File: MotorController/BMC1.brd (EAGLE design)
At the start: 92 x 50 mm, 58 parts, among them IC2 LP2950, IC3 MEGA8-AI, Q1 20MHz, U1 BTN8982TA, U2 BTN8982TA, U3 BTN8982TA, U4 TC77-5.0MCTTR, U5 MCP2561-E/SN

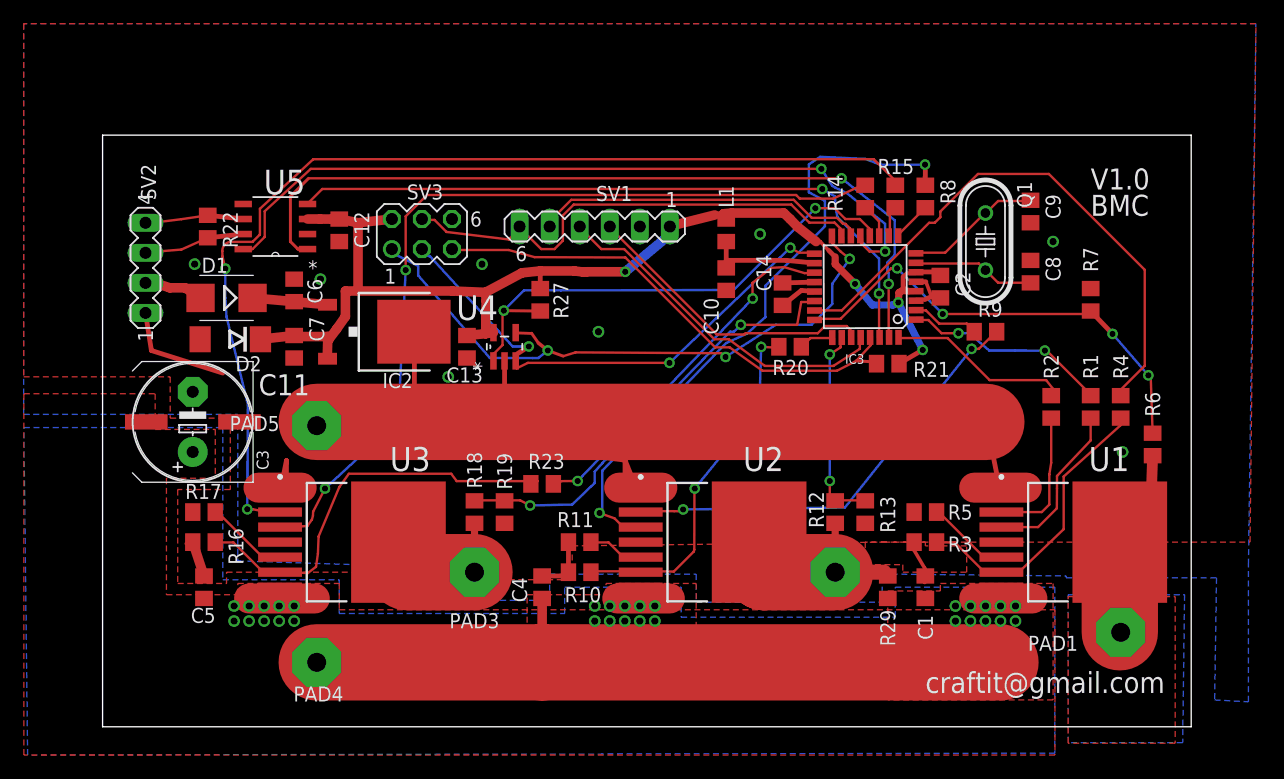
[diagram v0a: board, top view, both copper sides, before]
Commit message: Finished version 1.
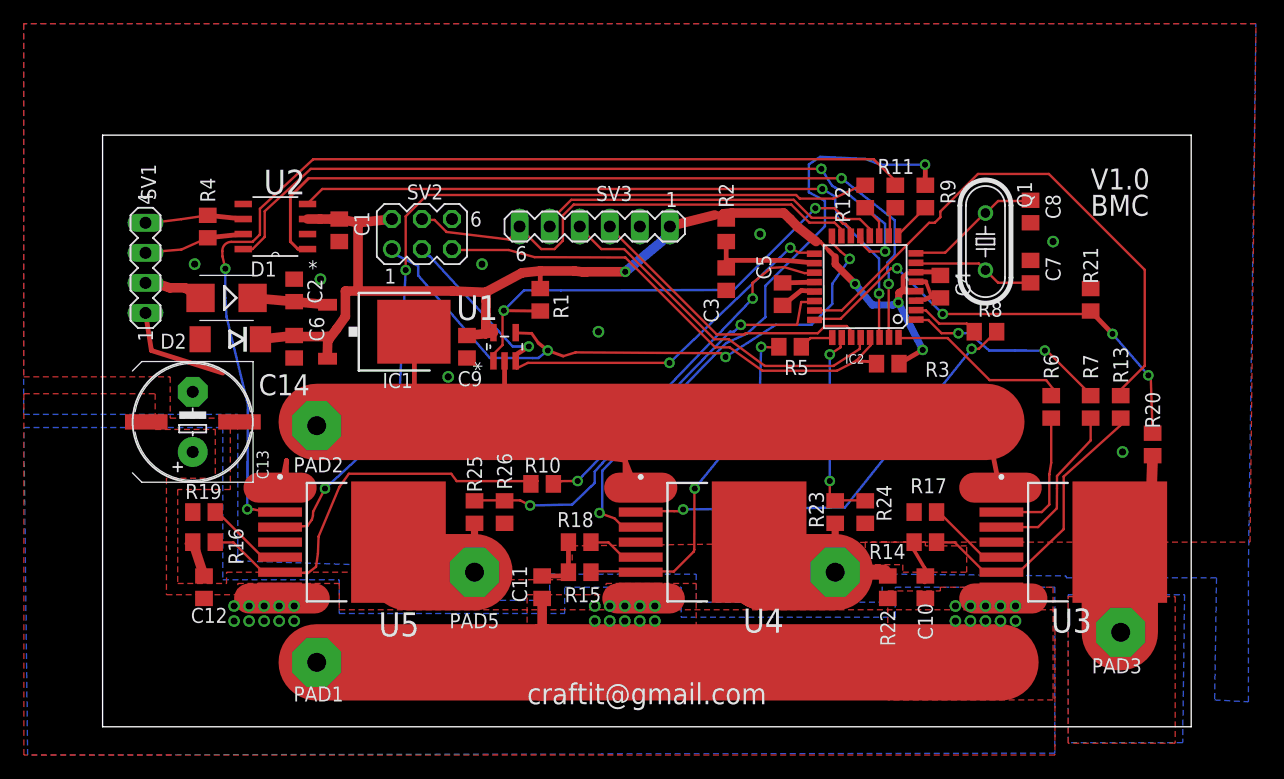
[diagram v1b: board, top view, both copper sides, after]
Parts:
- removed IC3: MEGA8-AI, atmel:TQFP32-08
- removed L1: 10uH, resistor:R0805
- removed R27, R29: 10k, resistor:R0805
- added IC1: LP2950, linear:DPACK
- added R24, R26: 1k, resistor:R0805
- added R25: 30k, resistor:R0805
- C1, C4, C5: value 0.1uf 40v -> 0.1uf
- C10, C12: value 0.1uf -> 0.1uf 40v
- C11: value (none) -> 0.1uf 40v; device resistor:E5-10,5 -> rcl:C0805
- C13: value 0.1uf -> 1000uF 50V; device rcl:C0805 -> rcl:UD-10X10_NICHICON
- C14: value 0.1uf -> 1000uf 50V; device rcl:C0805 -> resistor:E5-10,5
- C2: value 0.1uf -> 10uf 35V
- C3: value 1000uF 40V -> 0.1uf; device rcl:UD-10X10_NICHICON -> rcl:C0805
- C6: value 10uf 35V -> 2.2uf 10V
- C7: value 2.2uf 10V -> 18pf
- C9: value 18pf -> 0.1uf
- IC2: value LP2950 -> MEGA8-AI; device linear:DPACK -> atmel:TQFP32-08
- R10, R3: value 750R -> 10k
- R11, R5: value 100R -> 10k
- R12, R6: value 30k -> 10k
- R13, R7: value 1k -> 10k
- R14, R15: value 10k -> 750R
- R18: value 30k -> 100R
- R19: value 1k -> 100R
- R2: value 10k -> 10uH
- R20, R23: value 10k -> 30k
- R21: value 10k -> 1k
- R22: value 120R -> 10k
- R4: value 10k -> 120R
- SV1: device con-lstb:MA06-1 -> con-lstb:MA04-1
- SV2: device con-lstb:MA04-1 -> con-lstb:MA03-2
- SV3: device con-lstb:MA03-2 -> con-lstb:MA06-1
- U1: value BTN8982TA -> TC77-5.0MCTTR; device BTN8982TA:TO127P1500X440-8N-1 -> temp-tc77-5v:SOT95P290X145-5N
- U2: value BTN8982TA -> MCP2561-E/SN; device BTN8982TA:TO127P1500X440-8N-1 -> Microchip-MCP2561-E_SN:SOIC127P600X175-8N
- U4: value TC77-5.0MCTTR -> BTN8982TA; device temp-tc77-5v:SOT95P290X145-5N -> BTN8982TA:TO127P1500X440-8N-1
- U5: value MCP2561-E/SN -> BTN8982TA; device Microchip-MCP2561-E_SN:SOIC127P600X175-8N -> BTN8982TA:TO127P1500X440-8N-1
- moved R4 78.6 mm to (8.89, 42.3)
- moved PAD1 68.0 mm to (18.1, 5.45)
- moved R22 65.1 mm to (66.4, 11.8)
- moved C7 62.6 mm to (78.4, 38.5)
- moved U3 61.0 mm to (81.0, 15.6)
- moved R17 61.0 mm to (69.5, 18.1)
- moved C1 58.0 mm to (20.0, 42.0), turned to 270 degrees
- moved PAD3 54.8 mm to (86.0, 7.99)
- moved C5 54.8 mm to (57.5, 36.6), turned to 270 degrees
- moved C2 54.6 mm to (16.2, 36.9), turned to 90 degrees
- moved C14 51.0 mm to (7.62, 25.8), turned to 90 degrees
- moved U1 49.8 mm to (34.0, 32.1), turned to 90 degrees
- moved C9 49.0 mm to (30.8, 32.1), turned to 270 degrees
- moved R1 47.4 mm to (37.0, 36.1), turned to 90 degrees
- moved C3 46.7 mm to (52.7, 37.8), turned to 270 degrees
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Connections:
- removed net N$1 (its old number): R5.2, U1.5
- new net N$14: R19.2, U5.5
- net +7V: now also SV1.2; no longer SV2.2
- net 18V: now also C10.1, C11.1, C12.1, C13.+, C14.+, PAD1.1, R22.2, U4.7, U5.7; no longer C1.1, C11.+, C3.+, C4.1, C5.1, PAD4.1, R29.2, U1.7, U2.7
- net GND: now also C11.2, C13.-, C14.-, C3.2, C7.1, C9.2, IC1.2, IC2.21, IC2.3, IC2.5, PAD2.1, R14.1, R15.1, R18.1, R21.1, R24.1, R26.1, SV1.1, SV2.6, SV3.2, U1.2, U2.2, U4.1, U5.1; no longer C11.-, C13.2, C14.2, C3.-, C7.2, C9.1, IC2.2, IC3.21, IC3.3, IC3.5, PAD5.1, R10.1, R11.1, R13.1, R3.1, R5.1, R7.1, SV1.2, SV2.1, SV3.6, U1.1, U2.1, U4.2, U5.2
- net N$10: now also R8.2, U4.2; no longer R9.2, U2.2
- net N$11: now also IC2.25, R5.1; no longer IC3.25, R20.1
- net N$12: now also IC2.2, R8.1; no longer IC3.2, R9.1
- net N$13: now also PAD5.1, R25.2, U5.8; no longer PAD3.1, R18.2, U3.8
- net N$15: now also R12.2, U5.3; no longer R14.2, U3.3
- net N$16: now also R11.2, U5.2; no longer R15.2, U3.2
- net N$17: now also IC2.19, R10.1; no longer IC3.19, R23.1
- net N$18: now also IC2.22, R25.1, R26.2; no longer IC3.22, R18.1, R19.2
- net N$19: now also R4.1, SV1.4, U2.6; no longer R22.1, SV2.4, U5.6
- net N$2: now also PAD3.1, R20.2, U3.8; no longer PAD1.1, R6.2, U1.8
- net N$21: now also IC2.9, R9.1; no longer IC3.9, R8.1
- net N$22: now also IC2.26, R23.1, R24.2; no longer IC3.26, R12.1, R13.2
- net N$23: now also R4.2, SV1.3, U2.7; no longer R22.2, SV2.3, U5.7
- net N$25: now also IC2.13, U2.8; no longer IC3.13, U5.8
- net N$26: now also C2.1, IC1.1; no longer C6.1, IC2.1
- net N$27: now also C7.2, IC2.7; no longer C8.2, IC3.7
- net N$3: now also R7.2, U3.3; no longer R1.2, U1.3
- net N$31: now also C8.2, IC2.8; no longer C9.2, IC3.8
- net N$32: now also IC2.15, SV2.4, SV3.6; no longer IC3.15, SV1.6, SV3.4
- net N$33: now also IC2.32, R6.1; no longer IC3.32, R2.1
- net N$34: now also IC2.17, SV2.3, U1.3; no longer IC3.17, SV3.3, U4.3
- net N$36: now also R15.2, R5.2, U4.6; no longer R10.2, R20.2, U2.6
- net N$37: now also IC2.27, SV3.3; no longer IC3.27, SV1.3
- net N$38: now also R13.2, R14.2, U3.6; no longer R3.2, R4.2, U1.6
- net N$39: now also R10.2, U5.6; no longer R23.2, U3.6
- net N$4: now also R6.2, U3.2; no longer R2.2, U1.2
- net N$40: now also C3.1, IC2.18, R2.1; no longer C10.1, IC3.18, L1.1
- net N$41: now also IC2.28, SV3.4; no longer IC3.28, SV1.4
- net N$42: now also IC2.30, U2.4; no longer IC3.30, U5.4
- net N$43: now also IC2.31, U2.1; no longer IC3.31, U5.1
- net N$44: now also IC2.11, R12.1; no longer IC3.11, R14.1
- net N$45: now also IC2.10, R11.1; no longer IC3.10, R15.1
- net N$46: now also IC2.1, R7.1; no longer IC3.1, R1.1
- net N$49: now also IC2.14, SV3.5; no longer IC3.14, SV1.5
- net N$5: now also IC2.24, R20.1, R21.2; no longer IC3.24, R6.1, R7.2
- net N$50: now also IC2.12, R1.1, U1.1; no longer IC3.12, R27.1, U4.1
- net N$52: now also IC2.29, R3.2, SV2.5; no longer IC3.29, R21.2, SV3.5
- net N$54: now also C5.1, IC2.20; no longer C14.1, IC3.20
- net N$55: now also IC2.23, R13.1; no longer IC3.23, R4.1
- net N$6: now also IC2.16, SV2.1, U1.4; no longer IC3.16, SV3.1, U4.4
- net N$7: now also PAD4.1, R22.1, R23.2, U4.8; no longer PAD2.1, R12.2, R29.1, U2.8
- net N$8: now also R18.2, U4.5; no longer R11.2, U2.5
- net N$9: now also R9.2, U4.3; no longer R8.2, U2.3
- net VCC: now also C1.1, C4.1, C6.1, C9.1, IC1.3, IC2.4, IC2.6, R1.2, R2.2, R3.1, SV2.2, SV3.1, U1.5, U2.3; no longer C12.1, C13.1, C2.1, C7.1, IC2.3, IC3.4, IC3.6, L1.2, R21.1, R27.2, SV1.1, SV3.2, U4.5, U5.3
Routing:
- net N$14: track 0.00 -> 7.05 mm
- net N$1 (its old number): track 7.05 -> 0.00 mm
